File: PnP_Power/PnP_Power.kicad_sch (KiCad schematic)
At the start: 64 parts, among them J1 Barrel Jack 5mm x 2.5mm 54-00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, U7 VNH5019A-E, U8 LMS78_05-2.0R, U9 SN74LVC2G04DBVR

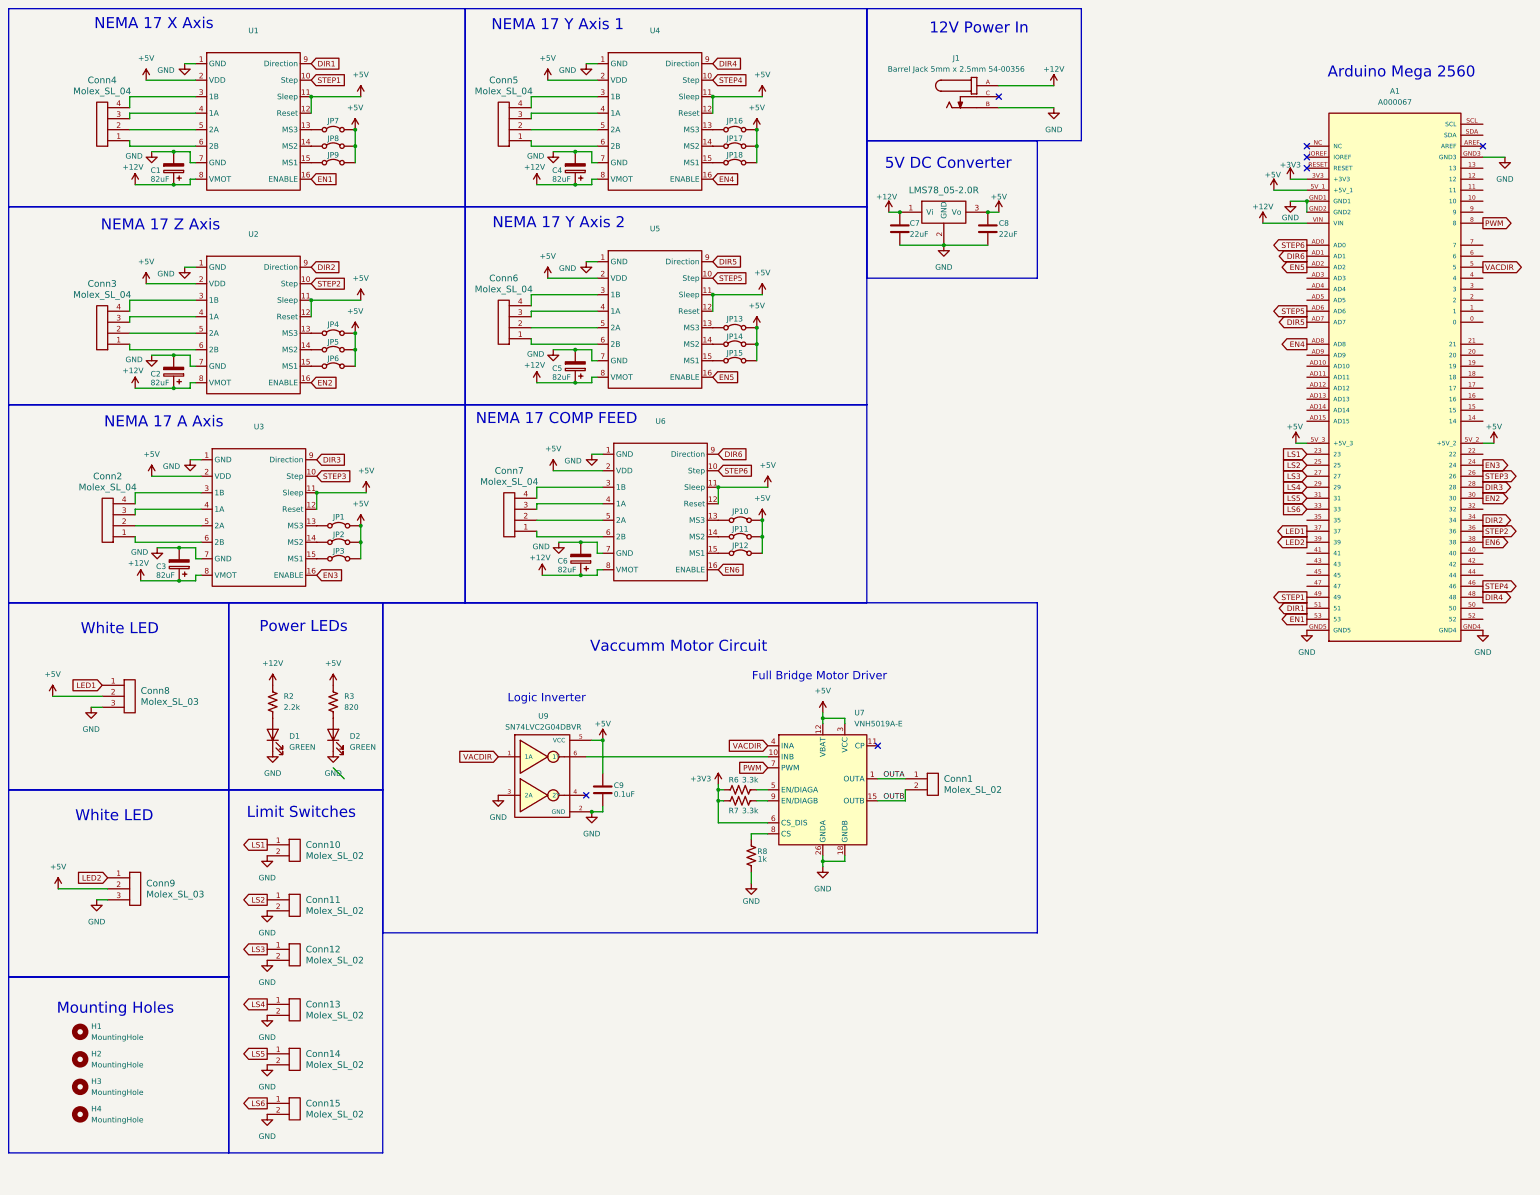
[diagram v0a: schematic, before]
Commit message: Many things
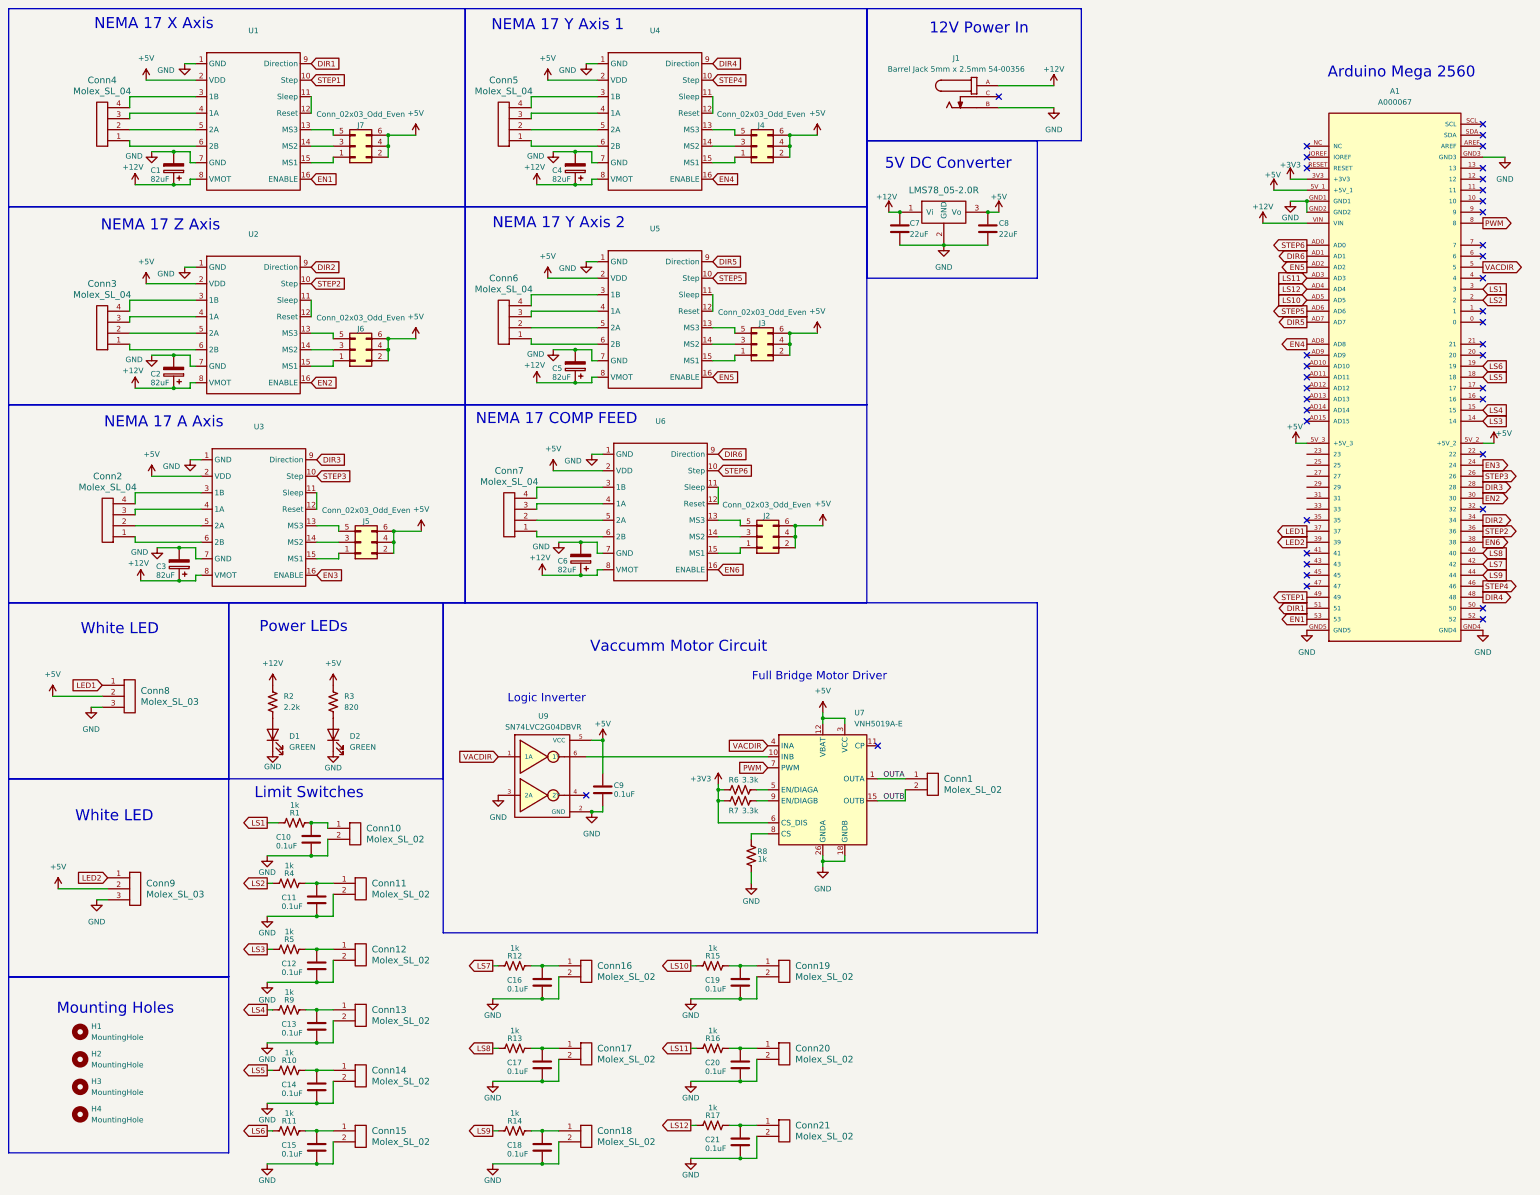
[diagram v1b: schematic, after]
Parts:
- removed JP1, JP10, JP11, JP12, JP13, JP14, JP15, JP16, JP17, JP18, JP2, JP3, JP4, JP5, JP6, JP7, JP8, JP9: Jumper_2_Bridged, Connector_PinHeader_2.54mm:PinHeader_1x02_P2.54mm_Vertical, symbol Jumper:Jumper_2_Bridged
- added C10, C11, C12, C13, C14, C15, C16, C17, C18, C19, C20, C21: 0.1uF, Capacitor_SMD:C_0603_1608Metric_Pad1.08x0.95mm_HandSolder, symbol Device:C
- added Conn16, Conn17, Conn18, Conn19, Conn20, Conn21: Molex_SL_02, MRDT_Connectors:MOLEX_SL_02_Horizontal, symbol MRDT_Connectors:Molex_SL_02
- added J2, J3, J4, J5, J6, J7: Conn_02x03_Odd_Even, Connector_PinHeader_2.54mm:PinHeader_2x03_P2.54mm_Vertical, symbol Connector_Generic:Conn_02x03_Odd_Even
- added R1, R10, R11, R12, R13, R14, R15, R16, R17, R4, R5, R9: 1k, Resistor_SMD:R_0603_1608Metric_Pad0.98x0.95mm_HandSolder, symbol Device:R_US
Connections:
- net +5V: now also J2.2 (Pin_2), J2.4 (Pin_4), J2.6 (Pin_6), J3.2 (Pin_2), J3.4 (Pin_4), J3.6 (Pin_6), J4.2 (Pin_2), J4.4 (Pin_4), J4.6 (Pin_6), J5.2 (Pin_2), J5.4 (Pin_4), J5.6 (Pin_6), J6.2 (Pin_2), J6.4 (Pin_4), J6.6 (Pin_6), J7.2 (Pin_2), J7.4 (Pin_4), J7.6 (Pin_6); no longer U1.11 (Sleep), U1.12 (Reset), U2.11 (Sleep), U2.12 (Reset), U3.11 (Sleep), U3.12 (Reset), U4.11 (Sleep), U4.12 (Reset), U5.11 (Sleep), U5.12 (Reset), U6.11 (Sleep), U6.12 (Reset)
- net GND: now also C10.2, C11.2, C12.2, C13.2, C14.2, C15.2, C16.2, C17.2, C18.2, C19.2, C20.2, C21.2, Conn16.2, Conn17.2, Conn18.2, Conn19.2, Conn20.2, Conn21.2
- net LS1: now also A1.3, R1.1; no longer A1.23, Conn10.1
- net LS2: now also A1.2, R4.1; no longer A1.25, Conn11.1
- net LS3: now also A1.14, R5.1; no longer A1.27, Conn12.1
- net LS4: now also A1.15, R9.1; no longer A1.29, Conn13.1
- net LS5: now also A1.18, R10.1; no longer A1.31, Conn14.1
- net LS6: now also A1.19, R11.1; no longer A1.33, Conn15.1
- net at U1.15 (MS1): now also J7.1 (Pin_1)
- net at U4.13 (MS3): now also J4.5 (Pin_5)
- net at U4.14 (MS2): now also J4.3 (Pin_3)
- net at U4.15 (MS1): now also J4.1 (Pin_1)
- net at U3.15 (MS1): now also J5.1 (Pin_1)
- net at U2.14 (MS2): now also J6.3 (Pin_3)
- net at U1.14 (MS2): now also J7.3 (Pin_3)
- net at U5.15 (MS1): now also J3.1 (Pin_1)
- net at U1.13 (MS3): now also J7.5 (Pin_5)
- net at U6.15 (MS1): now also J2.1 (Pin_1)
- net at U5.14 (MS2): now also J3.3 (Pin_3)
- net at U5.13 (MS3): now also J3.5 (Pin_5)
- net at U3.13 (MS3): now also J5.5 (Pin_5)
- net at U3.14 (MS2): now also J5.3 (Pin_3)
- net at U2.13 (MS3): now also J6.5 (Pin_5)
- net at U2.15 (MS1): now also J6.1 (Pin_1)
- net at U6.13 (MS3): now also J2.5 (Pin_5)
- net at U6.14 (MS2): now also J2.3 (Pin_3)
- net LS8: now reaches A1.40
- net LS8: now also R13.1
- net LS7: now reaches A1.42
- net LS7: now also R12.1
- net LS9: now reaches A1.44
- net LS9: now also R14.1
- net LS11: now reaches A1.AD3
- net LS11: now also R16.1
- net LS12: now reaches A1.AD4
- net LS12: now also R17.1
- net LS10: now reaches A1.AD5
- net LS10: now also R15.1
- new net: C11.1, Conn11.1, R4.2
- new net: C13.1, Conn13.1, R9.2
- new net: C17.1, Conn17.1, R13.2
- new net: C19.1, Conn19.1, R15.2
- new net: C21.1, Conn21.1, R17.2
- new net: C10.1, Conn10.1, R1.2
- new net: U4.11 (Sleep), U4.12 (Reset)
- new net: C12.1, Conn12.1, R5.2
- new net: C14.1, Conn14.1, R10.2
- new net: C15.1, Conn15.1, R11.2
- new net: C18.1, Conn18.1, R14.2
- new net: C16.1, Conn16.1, R12.2
- new net: C20.1, Conn20.1, R16.2
- new net: U2.11 (Sleep), U2.12 (Reset)
- new net: U3.11 (Sleep), U3.12 (Reset)
- new net: U5.11 (Sleep), U5.12 (Reset)
- new net: U6.11 (Sleep), U6.12 (Reset)
- new net: U1.11 (Sleep), U1.12 (Reset)
- no-connect marks 7 -> 39
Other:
- moved on the sheet: Conn10, Conn11, Conn12, Conn13, Conn14, Conn15
